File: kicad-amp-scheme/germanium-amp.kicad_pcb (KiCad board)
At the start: 2 copper layers, 83.5 x 51 mm, 27 parts, among them J1 Выход, J2 Кнтрл, J3 Пит, J4 Вход, Q1 ГT308, Q2 MП38, Q3 ГТ402, Q4 ГT404

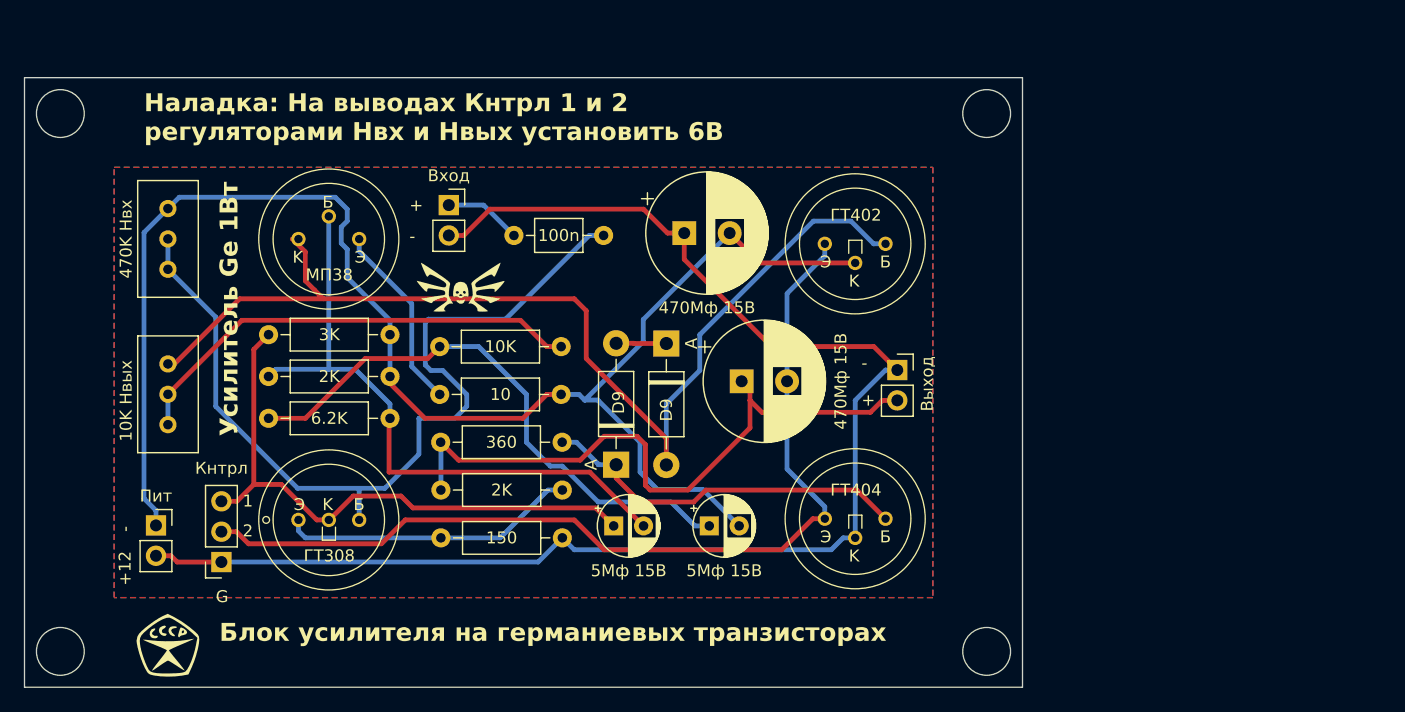
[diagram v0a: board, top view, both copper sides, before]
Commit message: Migrate to KiCad 8.0
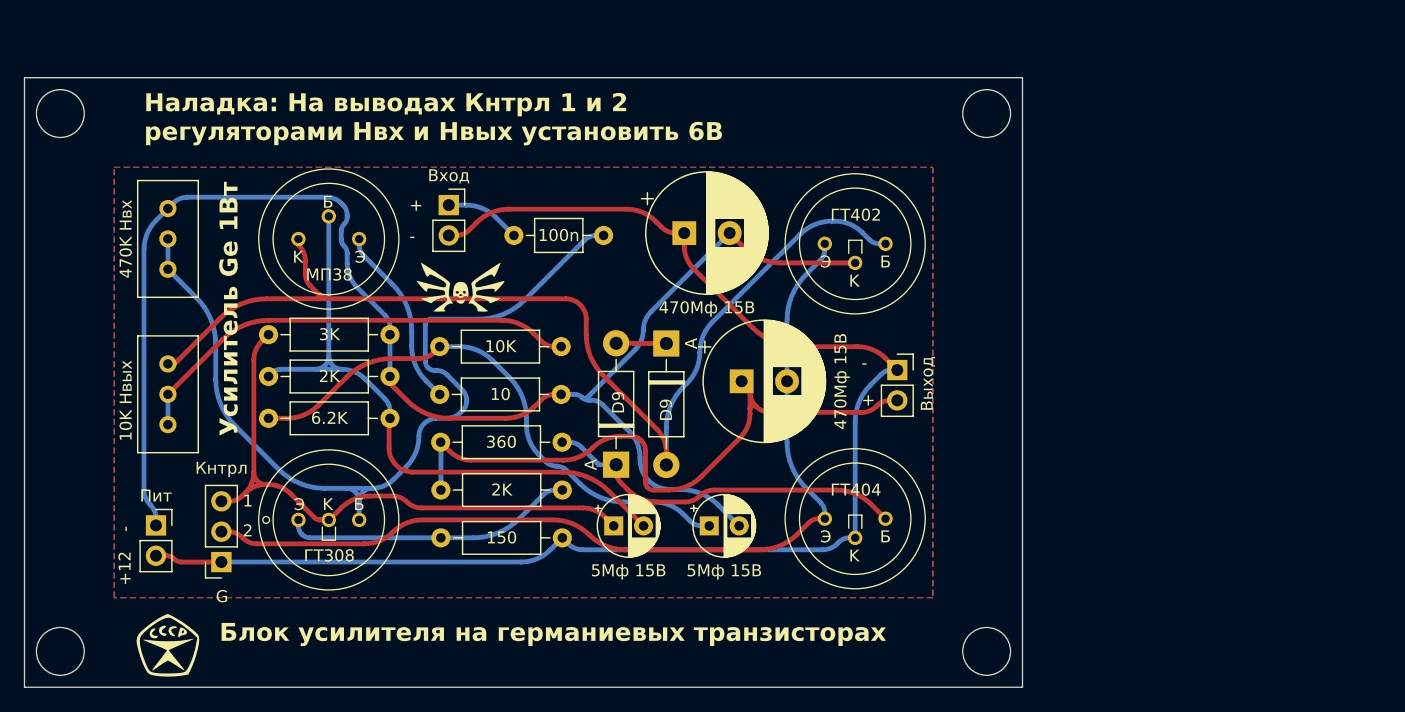
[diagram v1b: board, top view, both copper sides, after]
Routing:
- net Out -: track 121.8 -> 119.4 mm
- net -12V: track 127.8 -> 125.8 mm
- net Uh2: track 79.5 -> 77.7 mm
- net Net-(C4-Pad1): track 47.9 -> 46.2 mm
- net Uh1: track 49.5 -> 51.0 mm
- net Net-(D1-K): track 92.2 -> 91.0 mm
- net Net-(Q2-B): track 53.3 -> 54.1 mm
- net Net-(D2-A): track 31.2 -> 30.6 mm
- net Net-(Q2-E): track 15.8 -> 15.3 mm
- net Net-(R6-Pad2): track 38.9 -> 38.4 mm
